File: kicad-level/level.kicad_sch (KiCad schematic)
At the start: 6 parts, among them J1 Conn_01x01_Pin, J2 Conn_01x08_Pin, J3 Conn_01x01_Pin, U1 ULN2803A_C845537

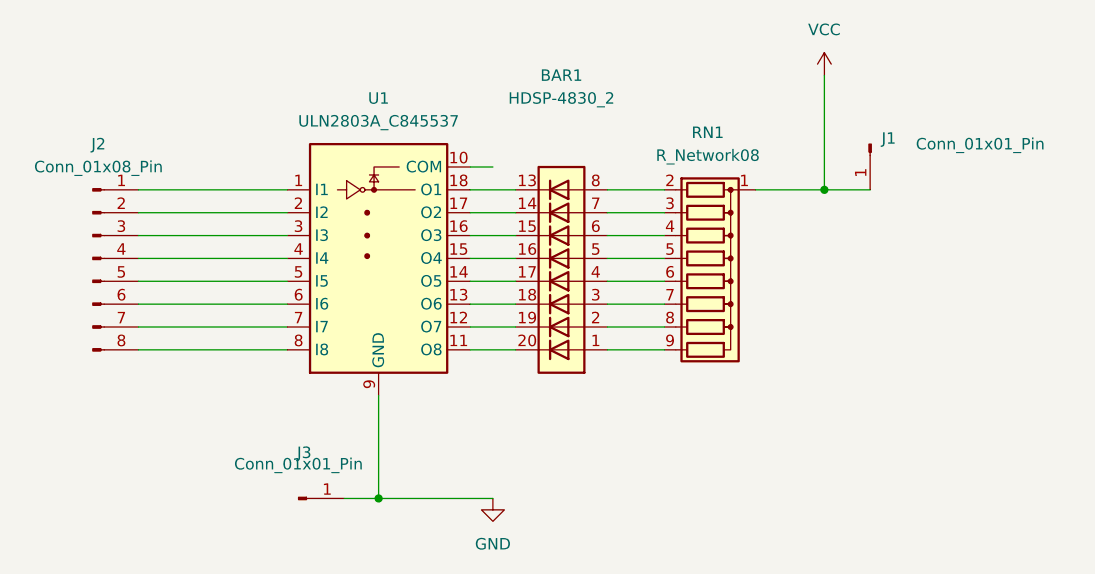
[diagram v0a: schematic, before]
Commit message: Revert "erreur pcb, com a la masse"
This reverts commit de789b6cb290ad22ceee4c73f03ad83cfbf3b982.
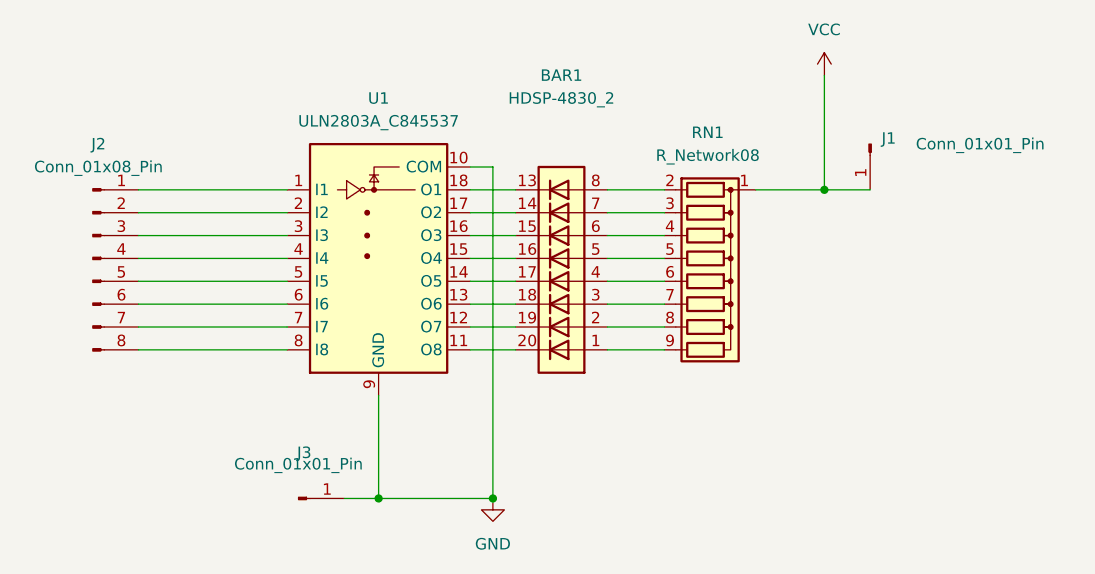
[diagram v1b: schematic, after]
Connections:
- net GND: now also U1.10 (COM)
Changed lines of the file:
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@@
 	(paper "A4")
+	(junction
+		(at 167.64 127)
+		(diameter 0)
+		(color 0 0 0 0)
+	)
 	(junction
 		(at 154.94 127)
@@
 		)
 		(stroke
+			(width 0)
+			(type default)
+		)
+	)
+	(wire
+		(pts
+			(xy 167.64 90.17) (xy 167.64 127)
+		)
+		(stroke
